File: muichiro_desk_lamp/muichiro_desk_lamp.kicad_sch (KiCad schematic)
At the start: 6 parts, among them J1 Conn_01x03_Pin, U1 ESP32-C3-DevKitM-1

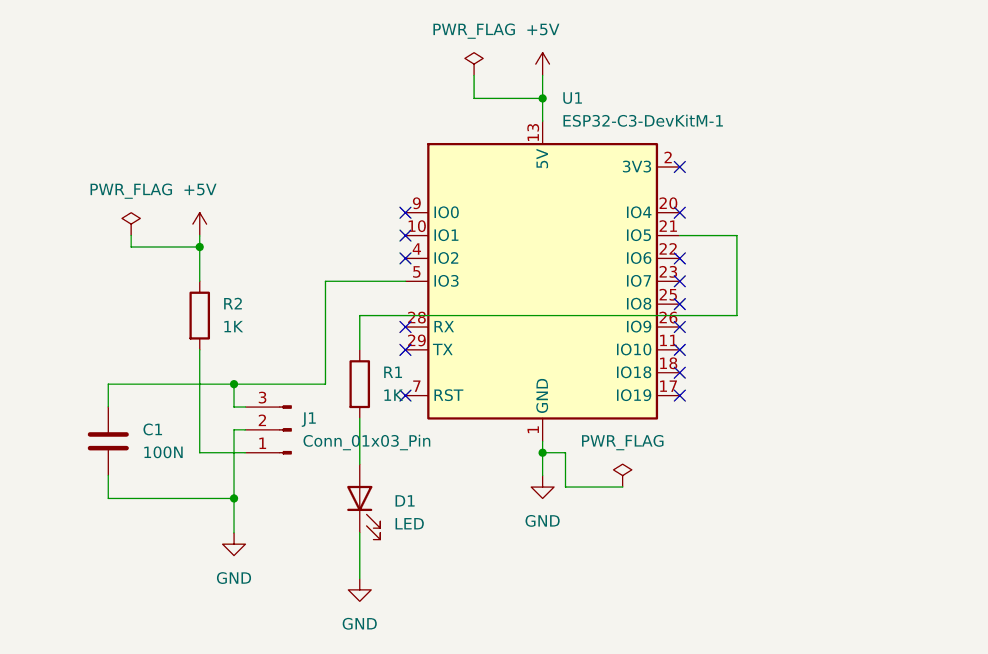
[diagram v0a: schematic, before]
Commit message: updated muichiro_desk_lamp
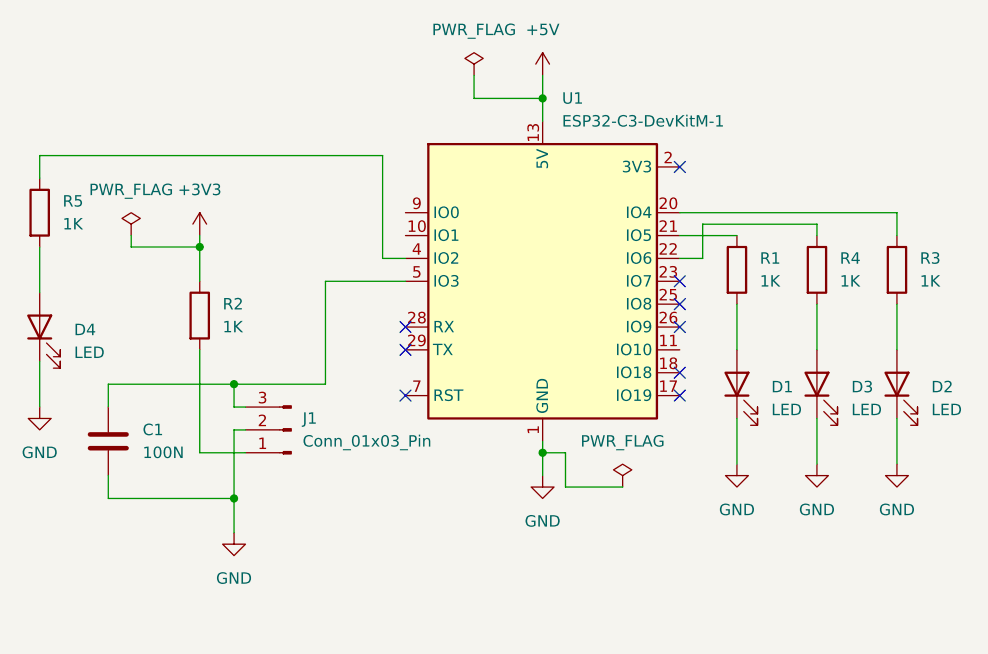
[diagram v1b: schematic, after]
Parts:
- added D2, D3, D4: LED, LED_SMD:LED_0805_2012Metric, symbol Device:LED
- added R3, R4, R5: 1K, Resistor_SMD:R_0805_2012Metric, symbol Device:R
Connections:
- net +5V: no longer R2.1
- net GND: now also D2.1 (K), D3.1 (K), D4.1 (K)
- net at U1.20 (IO4): now also R3.1
- net at U1.22 (IO6): now also R4.1
- net at U1.4 (IO2): now also R5.1
- new net: D2.2 (A), R3.2
- new net: D4.2 (A), R5.2
- new net: D3.2 (A), R4.2
- new net +3V3: R2.1
- no-connect marks 15 -> 9
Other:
- moved on the sheet: D1, R1
